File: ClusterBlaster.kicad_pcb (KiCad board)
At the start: 2 copper layers, 20 parts, among them J1 OBD2, J2 Cluster, SW1 UP, SW2 DOWN, SW3 ENTER, U1 LM339, U2 L7805, U3 ARDUINO_PRO_MINI

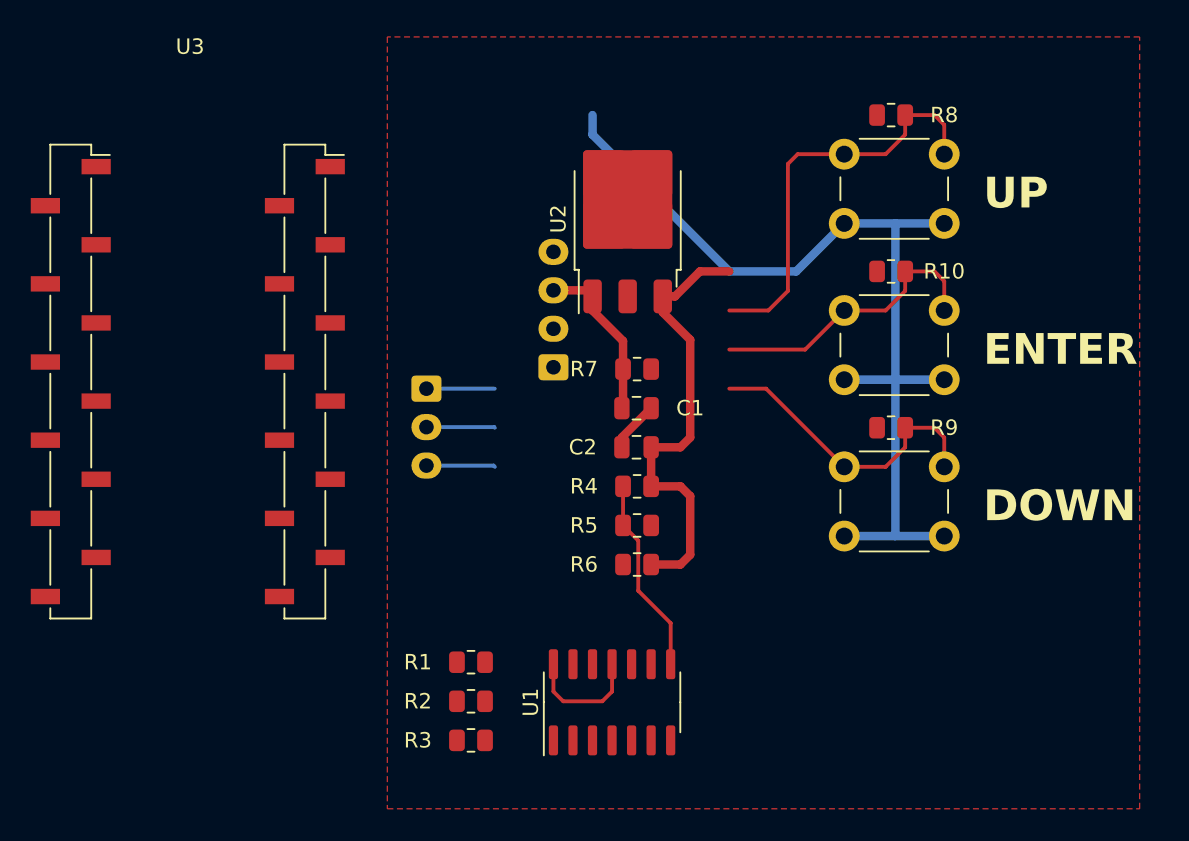
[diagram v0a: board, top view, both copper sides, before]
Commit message: Routed PCB
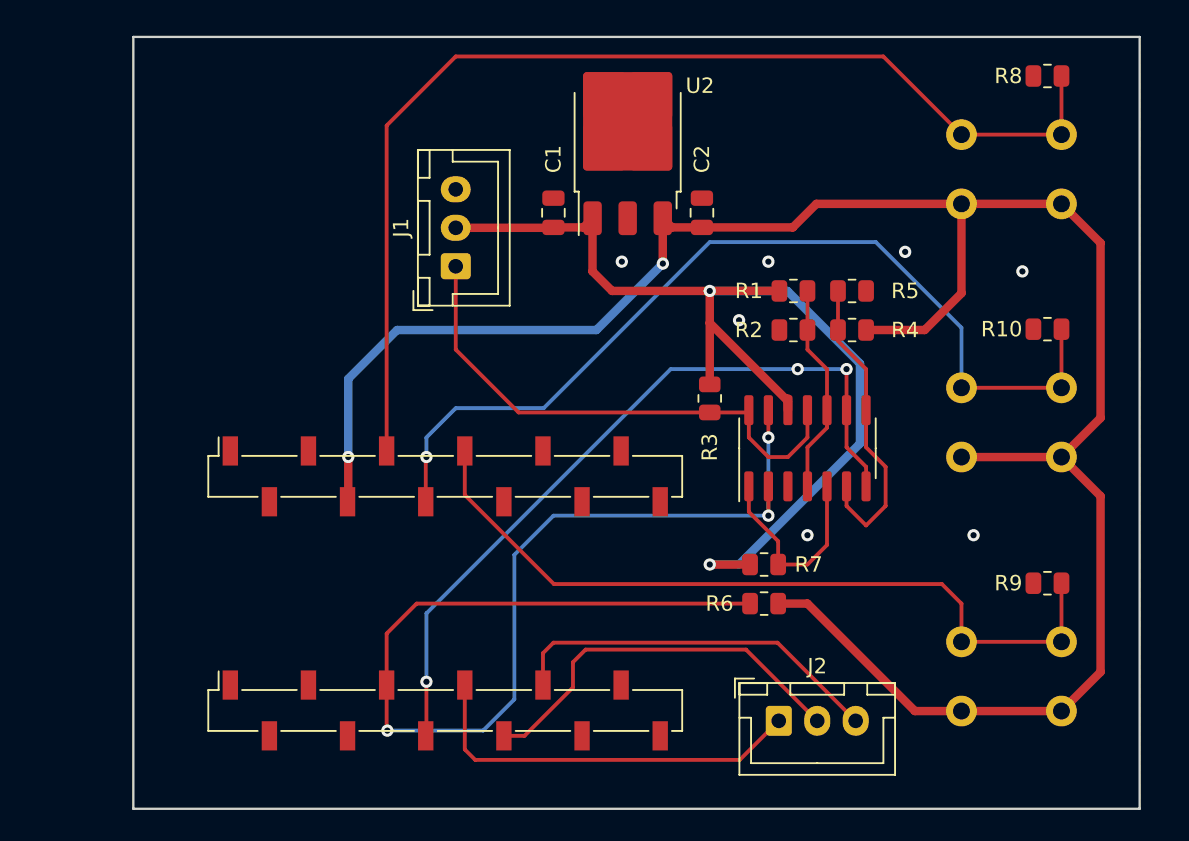
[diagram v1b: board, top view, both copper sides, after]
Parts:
- J1: footprint Connector_JST:JST_EH_B4B-EH-A_1x04_P2.50mm_Vertical -> Connector_JST:JST_XH_B3B-XH-A_1x03_P2.50mm_Vertical; moved to F.Cu
- J2: value Cluster -> Cluster Display; footprint Connector_JST:JST_EH_B3B-EH-A_1x03_P2.50mm_Vertical -> Connector_JST:JST_XH_B3B-XH-A_1x03_P2.50mm_Vertical; moved to F.Cu
- SW1, SW2, SW3: moved to B.Cu
- U3: value ARDUINO_PRO_MINI -> Arduino
- moved R2 32.0 mm to (160.4, 64.8), turned to 180 degrees
- moved R1 32.0 mm to (160.4, 62.2)
- moved J2 31.5 mm to (159.4, 90.2), turned to 0 degrees
- moved R3 27.1 mm to (154.9, 69.2), turned to -90 degrees
- moved U3 21.4 mm to (135.7, 81.7), turned to 90 degrees
- moved U1 20.8 mm to (161.3, 72.5)
- moved R5 20.7 mm to (164.2, 62.2)
- moved SW2 18.1 mm to (177.8, 85.0), turned to 180 degrees
- moved R4 17.3 mm to (164.2, 64.8)
- moved C2 15.8 mm to (154.4, 57.1), turned to 90 degrees
- moved R7 15.1 mm to (158.5, 80.0)
- moved SW3 15.0 mm to (177.8, 68.5), turned to 180 degrees
- moved R9 14.3 mm to (176.9, 81.2)
- moved SW1 14.2 mm to (177.8, 52.1), turned to 180 degrees
- moved C1 13.8 mm to (144.8, 57.1), turned to 90 degrees
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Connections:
- J1 pad 1: K-Line 2 -> K-Line
- J1 pad 2: K-Line -> +12V
- J1 pad 3: +12V -> GND
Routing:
- net RX: track 0.00 -> 75.6 mm, vias 0 -> 3
- net +12V: track 10.8 -> 72.5 mm, vias 0 -> 2
- net TX: track 0.00 -> 50.0 mm, vias 0 -> 2
- net 5V: track 92.1 -> 139.3 mm, vias 0 -> 2
- net BTN-UP: track 27.0 -> 72.8 mm
- net BTN-ENTER: track 19.0 -> 60.7 mm, vias 0 -> 1
- net BTN-DOWN: track 20.0 -> 50.9 mm
- net K-Line: track 7.89 -> 34.6 mm
- net CLOCK: track 4.44 -> 25.9 mm
- net DATA: track 4.46 -> 25.6 mm
- net ENABLE: track 4.48 -> 24.8 mm
- net Net-(U1A--): track 0.16 -> 13.8 mm
- net Net-(U1A-+): track 0.00 -> 13.4 mm
- net Net-(U1B--): track 12.8 -> 20.1 mm
- net GND: track 3.33 -> 0.00 mm, vias 0 -> 8
- added copper zone on B.Cu, net GND
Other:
- board outline added: 65.4 x 50.2 mm
